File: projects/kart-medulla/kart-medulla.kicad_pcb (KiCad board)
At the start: 2 copper layers, 68 x 60 mm, 59 parts, among them CN1 1990012, CN10 1990012, CN2 1990012, CN3 1990012, CN4 1990012, CN5 1990012, CN6 1990012, CN7 1990012, CN8 1990012, CN9 1990012, Q3 IRLZ44NPBF, Q4 BSS123_C5184436, U1 LM358DR, U13 MCP4922-E/SL, U14 MAX4660EUA+T, U19 L7805CDT_C20611927, U23 SSW-122-01-T-D, U24 SSW-122-01-T-S, U25 PCF8574T/3,518, U5 SN74LVC3G17DCTR

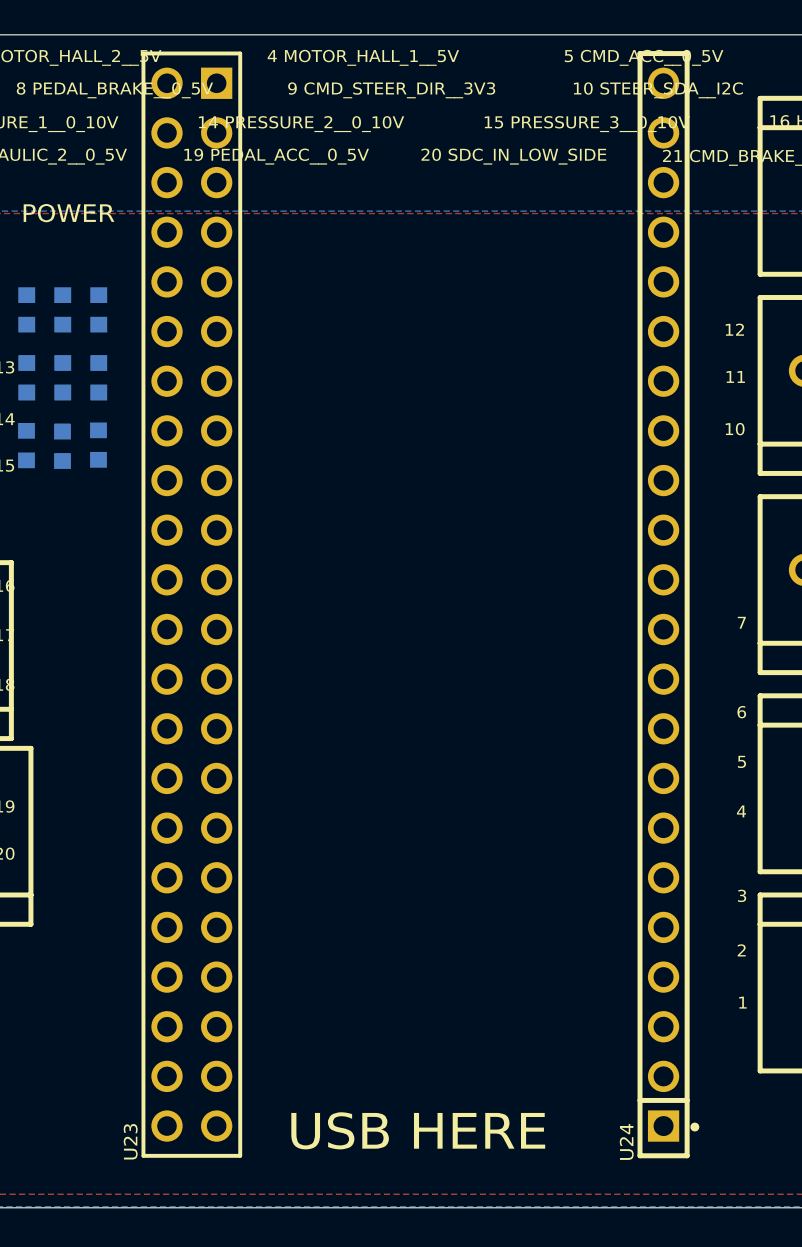
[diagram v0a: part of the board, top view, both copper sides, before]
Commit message: pcb ok
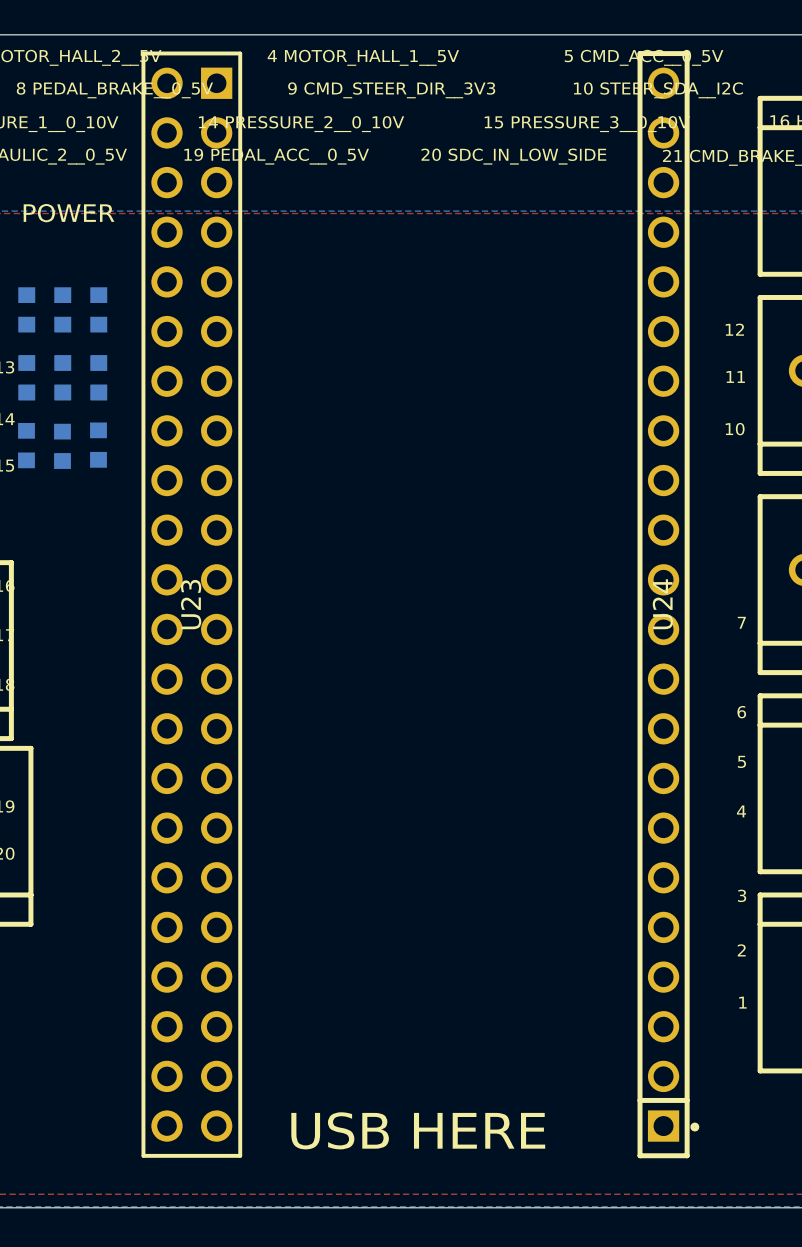
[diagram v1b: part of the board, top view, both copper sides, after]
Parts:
- U23: footprint HDR-TH_ESQ-122-59-G-D -> kart-medulla:HDR-TH_ESQ-122-59-G-D
- U24: footprint HDR-TH_ESQ-122-23-G-S -> kart-medulla:HDR-TH_ESQ-122-23-G-S
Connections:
- CN1 pad 1: /P1/HYDRAULIC_1__0_5V -> GND
- CN1 pad 2: +3V3 -> +12V
- CN1 pad 3: /P1/HYDRAULIC_2__0_5V -> GND
- CN10 pad 1: GND -> /P1/CMD_ACC__0_5V
- CN10 pad 2: /P1/EXP_P7 -> /P1/CMD_BRAKE__0_5V
- CN10 pad 3: /P1/EXP_P6 -> GND
- CN2 pad 1: /P1/PRESSURE_1__0_10V -> /P1/MOTOR_HALL_3__5V
- CN2 pad 2: /P1/PRESSURE_2__0_10V -> /P1/MOTOR_HALL_2__5V
- CN2 pad 3: /P1/PRESSURE_3__0_10V -> +5V_REG
- CN3 pad 1: /P1/CMD_STEER__PWM_3V3 -> /P1/CMD_STEER_DIR__3V3
- CN3 pad 2: /P1/PEDAL_BRAKE__0_5V -> /P1/EXP_P1
- CN3 pad 3: /P1/CMD_STEER_DIR__3V3 -> /P1/EXP_P2
- CN4 pad 1: /P1/SDA__I2C -> /P1/REVERSE_WIRE
- CN4 pad 2: /P1/SCL__I2C -> /P1/SDC_IN_LOW_SIDE
- CN4 pad 3: +3V3 -> /P1/CMD_STEER__PWM_3V3
- CN5 pad 1: /P1/PEDAL_ACC__0_5V -> /P1/HYDRAULIC_2__0_5V
- CN5 pad 2: /P1/SDC_IN_LOW_SIDE -> /P1/PRESSURE_3__0_10V
- CN5 pad 3: /P1/CMD_BRAKE__0_10V -> GND
- CN6 pad 1: GND -> /P1/PEDAL_ACC__0_5V
- CN6 pad 2: +12V -> /P1/PEDAL_BRAKE__0_5V
- CN6 pad 3: /P1/MOTOR_HALL_2__5V -> +3V3
- CN7 pad 1: /P1/MOTOR_HALL_1__5V -> /P1/PRESSURE_1__0_10V
- CN7 pad 2: /P1/MOTOR_HALL_3__5V -> /P1/PRESSURE_2__0_10V
- CN7 pad 3: /P1/CMD_ACC__0_5V -> /P1/MOTOR_HALL_1__5V
- CN8 pad 1: /P1/REVERSE_WIRE -> /P1/SDA__I2C
- CN8 pad 2: /P1/EXP_P2 -> /P1/BUZZER
- CN8 pad 3: /P1/EXP_P1 -> /P1/EXP_P3
- CN9 pad 1: /P1/EXP_P5 -> /P1/SCL__I2C
- CN9 pad 2: /P1/EXP_P4 -> /P1/HYDRAULIC_1__0_5V
- CN9 pad 3: /P1/EXP_P3 -> /P1/EXP_P4
- U25 pad 10: /P1/EXP_P5 -> unconnected-(U25-P5-Pad10)
- U25 pad 11: /P1/EXP_P6 -> unconnected-(U25-P6-Pad11)
- U25 pad 12: /P1/EXP_P7 -> unconnected-(U25-P7-Pad12)
